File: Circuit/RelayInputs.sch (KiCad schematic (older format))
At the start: 6 parts, among them K301 Meisei-m4-24h, K302 Meisei-m4-24h, K303 Meisei-m4-24h, K304 Meisei-m4-24h, K305 Meisei-m4-24h, K306 Meisei-m4-24h

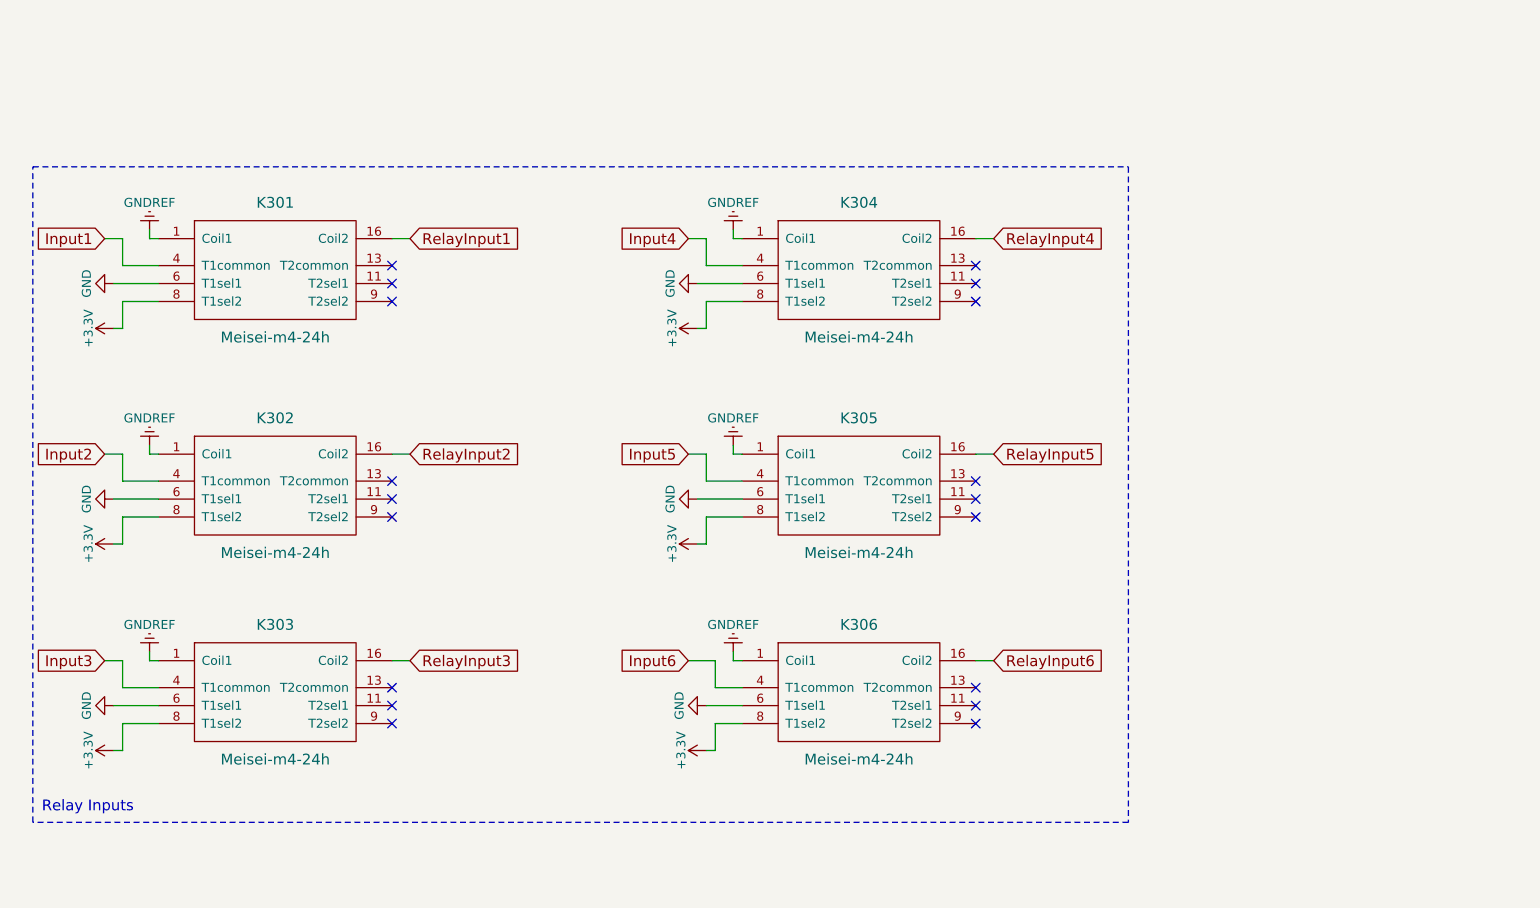
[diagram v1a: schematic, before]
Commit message: Additional PCB work
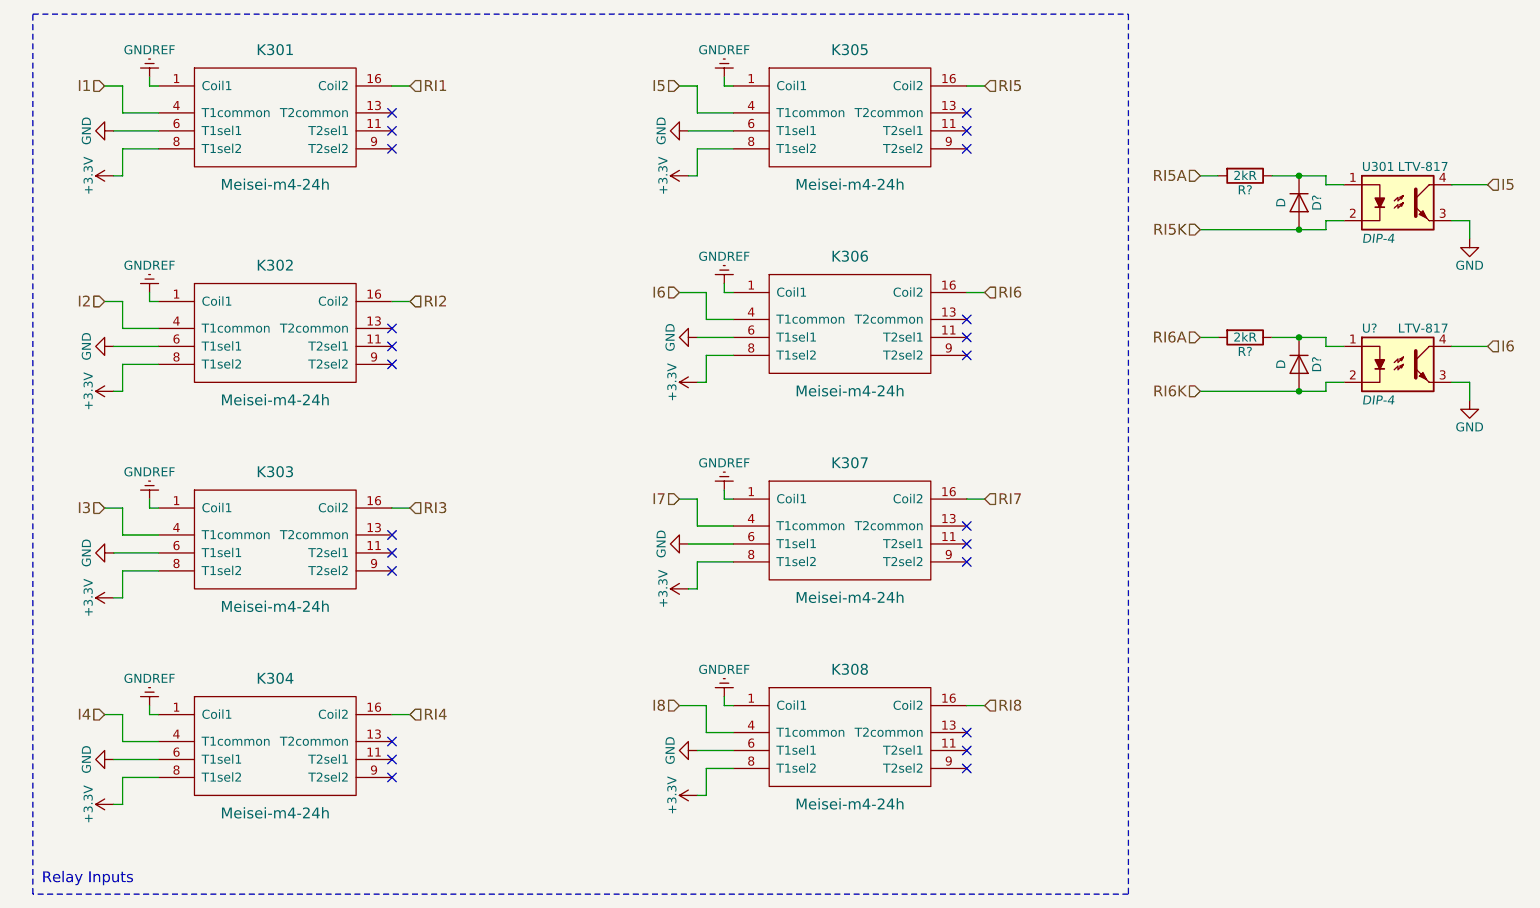
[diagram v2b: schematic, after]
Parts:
- added D? (x2): D, symbol D
- added K307, K308: Meisei-m4-24h, Meisei:Meisei-m4-24h, symbol Meisei-m4-24h
- added R? (x2): 2kR, symbol R
- added U301, U?: LTV-817, DIP-4, symbol LTV-817
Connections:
- net +3V3: now also K307.8 (T1sel2), K308.8 (T1sel2)
- net GND: now also K307.6 (T1sel1), K308.6 (T1sel1), U301.3, U?.3
- net GNDREF: now also K307.1 (Coil1), K308.1 (Coil1)
- net Input1 renamed I1
- net Input2 renamed I2
- net Input3 renamed I3
- net Input4 renamed I4
- net Input5 renamed I5
- net I5: now also U301.4
- net Input6 renamed I6
- net I6: now also U?.4
- net RelayInput1 renamed RI1
- net RelayInput2 renamed RI2
- net RelayInput3 renamed RI3
- net RelayInput4 renamed RI4
- net RelayInput5 renamed RI5
- net RelayInput6 renamed RI6
- new net: D?.1 (K), R?.1, U301.1
- new net: D?.1 (K), R?.1, U?.1
- new net I7: K307.4 (T1common)
- new net I8: K308.4 (T1common)
- new net RI5A: R?.2
- new net RI5K: D?.2 (A), U301.2
- new net RI6A: R?.2
- new net RI6K: D?.2 (A), U?.2
- new net RI7: K307.16 (Coil2)
- new net RI8: K308.16 (Coil2)
- no-connect marks 18 -> 24
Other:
- moved on the sheet: K301, K302, K303, K304, K305, K306
